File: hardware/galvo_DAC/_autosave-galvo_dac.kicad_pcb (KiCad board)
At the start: 2 copper layers, 43.2 x 40.6 mm, 33 parts, among them K1 CONN_3, K2 CONN_3, K3 CONN_3, P1 CONN_9, P2 CONN_2, P3 CONN_2, P4 CONN_2, Q1 PZT2222A, Q2 PZT2222A, Q3 PZT2222A, U1 LM358, U2 LM358, U3 MCP4822

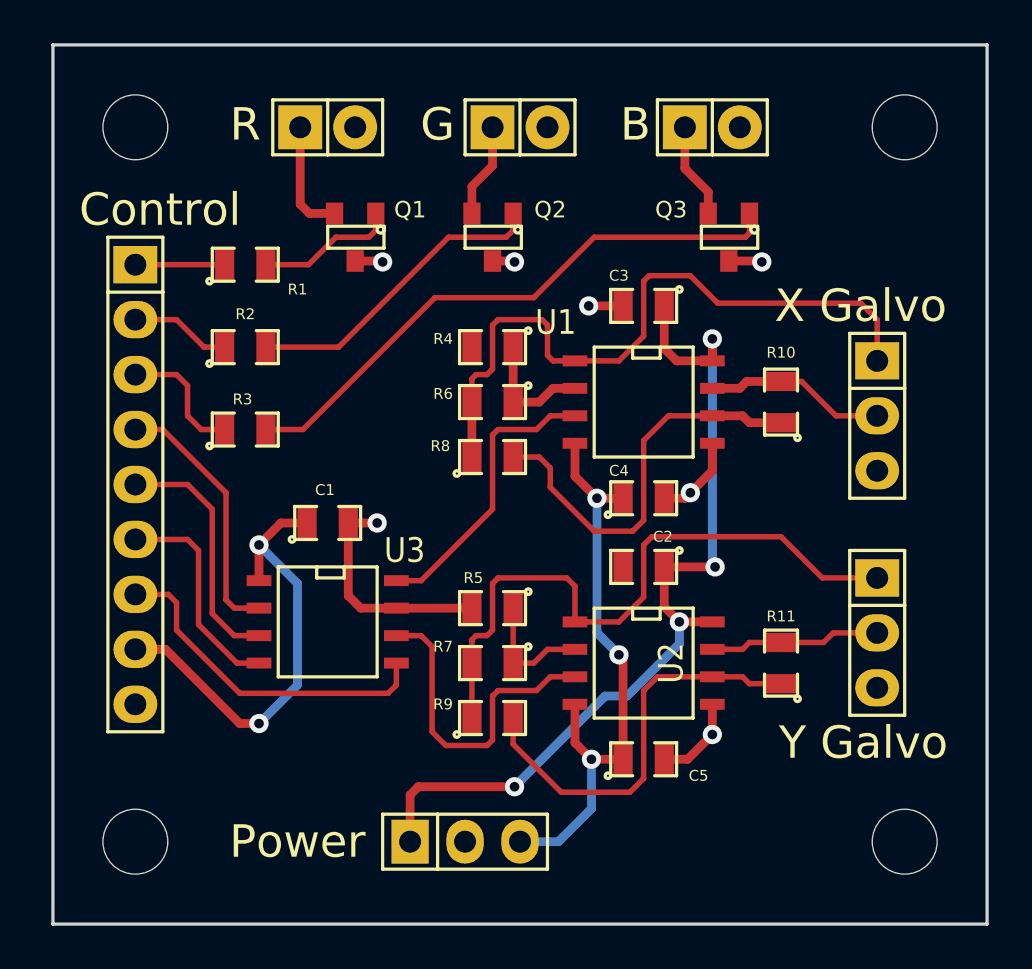
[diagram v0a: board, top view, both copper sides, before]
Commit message: Finished PCB, sent to Fab
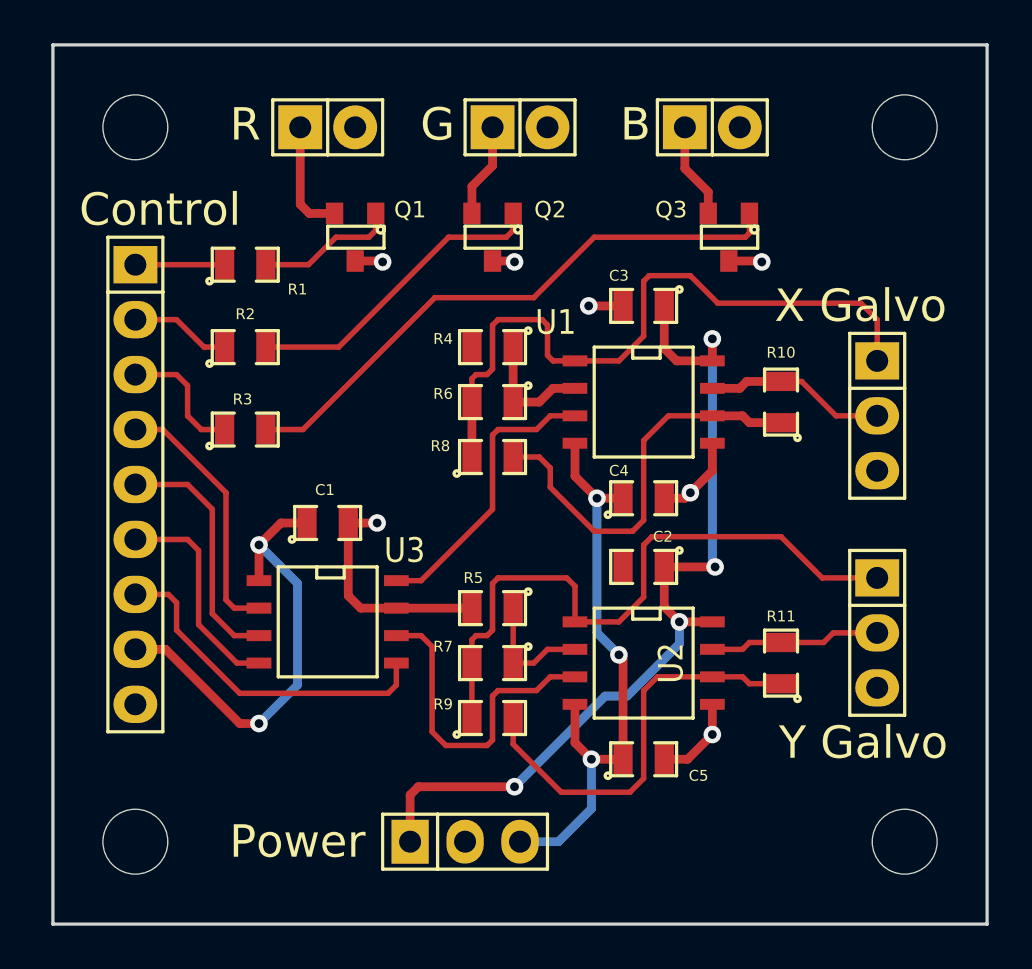
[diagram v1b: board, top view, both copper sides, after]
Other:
- rule via_min_size: 0.889 -> 0.3302
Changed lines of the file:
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@@
     (via_size 0.889)
     (via_drill 0.635)
-    (via_min_size 0.889)
+    (via_min_size 0.3302)
     (via_min_drill 0.508)
+    (user_via 0.8128 0.4046)
     (uvia_size 0.508)
     (uvia_drill 0.127)
@@
   (segment (start 157.48 115.57) (end 158.877 115.57) (width 0.4064) (layer F.Cu) (net 1))
   (segment (start 163.195 110.744) (end 163.195 112.395) (width 0.4064) (layer F.Cu) (net 1))
-  (via (at 163.195 110.744) (size 0.889) (layers F.Cu B.Cu) (net 1))
+  (via (at 163.195 110.744) (size 0.8128) (drill 0.4046) (layers F.Cu B.Cu) (net 1))
   (segment (start 164.973 112.522) (end 163.195 110.744) (width 0.4064) (layer B.Cu) (net 1))
   (segment (start 164.973 117.221) (end 164.973 112.522) (width 0.4064) (layer B.Cu) (net 1))
   (segment (start 163.195 118.999) (end 164.973 117.221) (width 0.4064) (layer B.Cu) (net 1))
-  (via (at 163.195 118.999) (size 0.889) (layers F.Cu B.Cu) (net 1))
+  (via (at 163.195 118.999) (size 0.8128) (drill 0.4046) (layers F.Cu B.Cu) (net 1))
   (segment (start 162.306 118.999) (end 163.195 118.999) (width 0.4064) (layer F.Cu) (net 1))
   (segment (start 158.877 115.57) (end 162.306 118.999) (width 0.4064) (layer F.Cu) (net 1))
   (segment (start 167.3225 109.728) (end 168.656 109.728) (width 0.4064) (layer F.Cu) (net 2))
-  (via (at 168.656 109.728) (size 0.889) (layers F.Cu B.Cu) (net 2))
+  (via (at 168.656 109.728) (size 0.8128) (drill 0.4046) (layers F.Cu B.Cu) (net 2))
   (segment (start 169.545 113.665) (end 167.894 113.665) (width 0.4064) (layer F.Cu) (net 2))
   (segment (start 167.3225 113.0935) (end 167.3225 109.728) (width 0.4064) (layer F.Cu) (net 2))
@@
   (segment (start 184.912 97.61982) (end 186.39282 97.61982) (width 0.4064) (layer F.Cu) (net 2))
   (segment (start 186.436 97.663) (end 186.563 97.663) (width 0.4064) (layer B.Cu) (net 2))
-  (via (at 186.436 97.663) (size 0.889) (layers F.Cu B.Cu) (net 2))
+  (via (at 186.436 97.663) (size 0.8128) (drill 0.4046) (layers F.Cu B.Cu) (net 2))
   (segment (start 186.39282 97.61982) (end 186.436 97.663) (width 0.4064) (layer F.Cu) (net 2))
   (segment (start 167.64 97.61982) (end 168.86682 97.61982) (width 0.4064) (layer F.Cu) (net 2))
-  (via (at 168.91 97.663) (size 0.889) (layers F.Cu B.Cu) (net 2))
+  (via (at 168.91 97.663) (size 0.8128) (drill 0.4046) (layers F.Cu B.Cu) (net 2))
   (segment (start 168.86682 97.61982) (end 168.91 97.663) (width 0.4064) (layer F.Cu) (net 2))
   (segment (start 173.99 97.61982) (end 174.96282 97.61982) (width 0.4064) (layer F.Cu) (net 2))
-  (via (at 175.006 97.663) (size 0.889) (layers F.Cu B.Cu) (net 2))
+  (via (at 175.006 97.663) (size 0.8128) (drill 0.4046) (layers F.Cu B.Cu) (net 2))
   (segment (start 174.96282 97.61982) (end 175.006 97.663) (width 0.4064) (layer F.Cu) (net 2))
   (segment (start 180.0225 99.695) (end 178.435 99.695) (width 0.4064) (layer F.Cu) (net 2))
-  (via (at 178.435 99.695) (size 0.889) (layers F.Cu B.Cu) (net 2))
-  (via (at 183.134 108.331) (size 0.889) (layers F.Cu B.Cu) (net 2))
+  (via (at 178.435 99.695) (size 0.8128) (drill 0.4046) (layers F.Cu B.Cu) (net 2))
+  (via (at 183.134 108.331) (size 0.8128) (drill 0.4046) (layers F.Cu B.Cu) (net 2))
   (segment (start 181.9275 108.585) (end 182.88 108.585) (width 0.4064) (layer F.Cu) (net 2))
   (segment (start 184.15 107.315) (end 184.15 106.045) (width 0.4064) (layer F.Cu) (net 2))
   (segment (start 182.88 108.585) (end 183.134 108.331) (width 0.4064) (layer F.Cu) (net 2))
   (segment (start 183.134 108.331) (end 184.15 107.315) (width 0.4064) (layer F.Cu) (net 2))
-  (via (at 184.15 119.507) (size 0.889) (layers F.Cu B.Cu) (net 2))
+  (via (at 184.15 119.507) (size 0.8128) (drill 0.4046) (layers F.Cu B.Cu) (net 2))
   (segment (start 181.9275 120.65) (end 183.007 120.65) (width 0.4064) (layer F.Cu) (net 2))
   (segment (start 184.15 119.507) (end 184.15 118.11) (width 0.4064) (layer F.Cu) (net 2))
@@
   (segment (start 181.9275 111.76) (end 184.277 111.76) (width 0.4064) (layer F.Cu) (net 3))
   (segment (start 184.15 101.219) (end 184.15 102.235) (width 0.4064) (layer F.Cu) (net 3))
-  (via (at 184.15 101.219) (size 0.889) (layers F.Cu B.Cu) (net 3))
+  (via (at 184.15 101.219) (size 0.8128) (drill 0.4046) (layers F.Cu B.Cu) (net 3))
   (segment (start 184.15 111.633) (end 184.15 101.219) (width 0.4064) (layer B.Cu) (net 3))
   (segment (start 184.277 111.76) (end 184.15 111.633) (width 0.4064) (layer B.Cu) (net 3))
-  (via (at 184.277 111.76) (size 0.889) (layers F.Cu B.Cu) (net 3))
+  (via (at 184.277 111.76) (size 0.8128) (drill 0.4046) (layers F.Cu B.Cu) (net 3))
   (segment (start 170.18 124.46) (end 170.18 122.301) (width 0.4064) (layer F.Cu) (net 3))
-  (via (at 182.626 114.3) (size 0.889) (layers F.Cu B.Cu) (net 3))
+  (via (at 182.626 114.3) (size 0.8128) (drill 0.4046) (layers F.Cu B.Cu) (net 3))
   (segment (start 182.626 115.316) (end 182.626 114.3) (width 0.4064) (layer B.Cu) (net 3))
   (segment (start 180.213 117.729) (end 182.626 115.316) (width 0.4064) (layer B.Cu) (net 3))
   (segment (start 179.197 117.729) (end 180.213 117.729) (width 0.4064) (layer B.Cu) (net 3))
   (segment (start 175.006 121.92) (end 179.197 117.729) (width 0.4064) (layer B.Cu) (net 3))
-  (via (at 175.006 121.92) (size 0.889) (layers F.Cu B.Cu) (net 3))
+  (via (at 175.006 121.92) (size 0.8128) (drill 0.4046) (layers F.Cu B.Cu) (net 3))
   (segment (start 170.561 121.92) (end 175.006 121.92) (width 0.4064) (layer F.Cu) (net 3))
   (segment (start 170.18 122.301) (end 170.561 121.92) (width 0.4064) (layer F.Cu) (net 3))
@@
   (segment (start 182.499 102.235) (end 184.15 102.235) (width 0.4064) (layer F.Cu) (net 3))
   (segment (start 180.0225 120.65) (end 180.0225 116.0145) (width 0.4064) (layer F.Cu) (net 4))
-  (via (at 178.816 108.585) (size 0.889) (layers F.Cu B.Cu) (net 4))
+  (via (at 178.816 108.585) (size 0.8128) (drill 0.4046) (layers F.Cu B.Cu) (net 4))
   (segment (start 178.816 114.808) (end 178.816 108.585) (width 0.4064) (layer B.Cu) (net 4))
   (segment (start 179.832 115.824) (end 178.816 114.808) (width 0.4064) (layer B.Cu) (net 4))
-  (via (at 179.832 115.824) (size 0.889) (layers F.Cu B.Cu) (net 4))
+  (via (at 179.832 115.824) (size 0.8128) (drill 0.4046) (layers F.Cu B.Cu) (net 4))
   (segment (start 180.0225 116.0145) (end 179.832 115.824) (width 0.4064) (layer F.Cu) (net 4))
   (segment (start 175.26 124.46) (end 177.038 124.46) (width 0.4064) (layer B.Cu) (net 4))
-  (via (at 178.562 120.65) (size 0.889) (layers F.Cu B.Cu) (net 4))
+  (via (at 178.562 120.65) (size 0.8128) (drill 0.4046) (layers F.Cu B.Cu) (net 4))
   (segment (start 178.562 122.936) (end 178.562 120.65) (width 0.4064) (layer B.Cu) (net 4))
   (segment (start 177.038 124.46) (end 178.562 122.936) (width 0.4064) (layer B.Cu) (net 4))
